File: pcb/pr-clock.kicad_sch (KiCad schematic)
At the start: 2 parts, among them U1 TM1637_C2962580

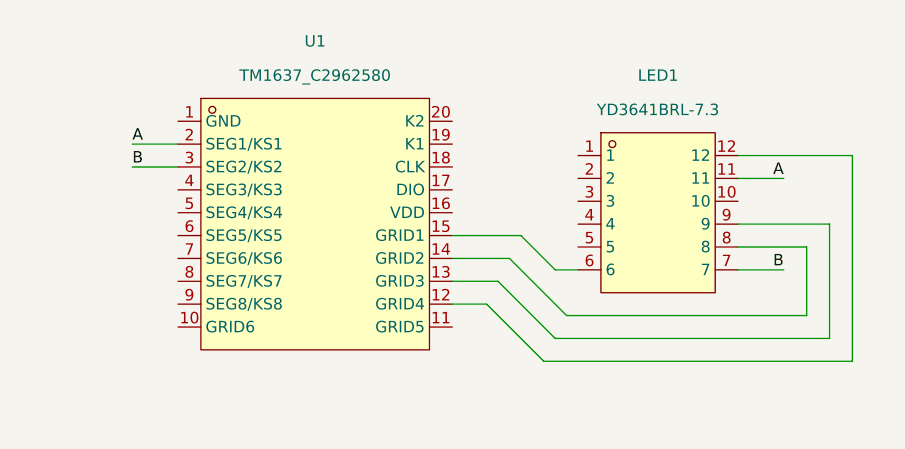
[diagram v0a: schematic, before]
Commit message: update
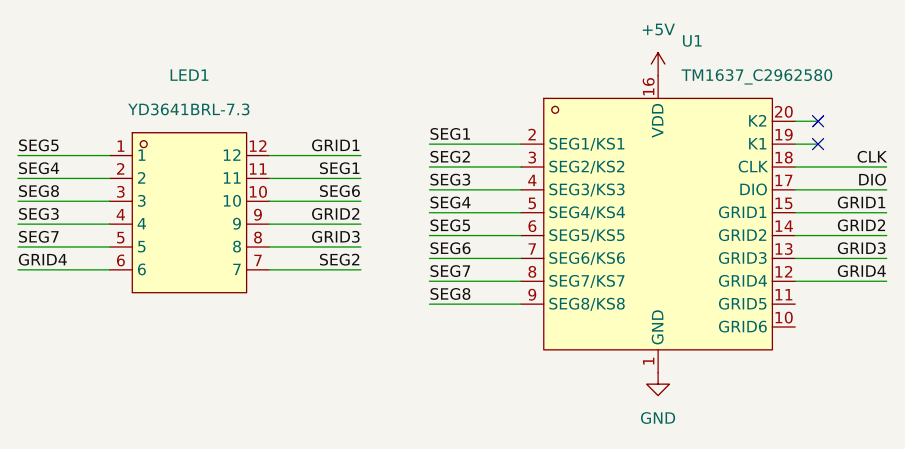
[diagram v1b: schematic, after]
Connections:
- net GND: now reaches U1.1 (GND)
- net GRID1: now reaches LED1.12
- net GRID1: now also U1.15 (GRID1); no longer U1.12 (GRID4)
- net GRID2: now reaches LED1.9
- net GRID2: now also U1.14 (GRID2); no longer U1.13 (GRID3)
- net GRID3: now reaches LED1.8
- net GRID3: now also U1.13 (GRID3); no longer U1.14 (GRID2)
- net GRID4: now reaches LED1.6
- net GRID4: now also U1.12 (GRID4); no longer U1.15 (GRID1)
- net +5V: now reaches U1.16 (VDD)
- net DIO: now reaches U1.17 (DIO)
- net CLK: now reaches U1.18 (CLK)
- net SEG3: now reaches U1.4 (SEG3/KS3)
- net SEG3: now also LED1.4
- net SEG4: now reaches U1.5 (SEG4/KS4)
- net SEG4: now also LED1.2
- net SEG5: now reaches U1.6 (SEG5/KS5)
- net SEG5: now also LED1.1
- net SEG6: now reaches U1.7 (SEG6/KS6)
- net SEG6: now also LED1.10
- net SEG7: now reaches U1.8 (SEG7/KS7)
- net SEG7: now also LED1.5
- net SEG8: now reaches U1.9 (SEG8/KS8)
- net SEG8: now also LED1.3
- net A renamed SEG1
- net B renamed SEG2
- no-connect marks 0 -> 2
